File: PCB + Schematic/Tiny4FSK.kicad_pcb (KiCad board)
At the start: 4 copper layers, 30.9 x 65.8 mm, 81 parts, among them IC1 SI4063, J1 SWD, J2 GPIO, J3 USBC, J4 OPTIONAL, J5 I2C, J6 Power, J7 SPI, SW1 RST, SW2 BATT PWR, U1 BME280, U2 MAX-M10S, U3 Linear Step-Down, U4 ATSAMD21G18A-A, U5 TCXO MCU, U6 TPS61200DRC

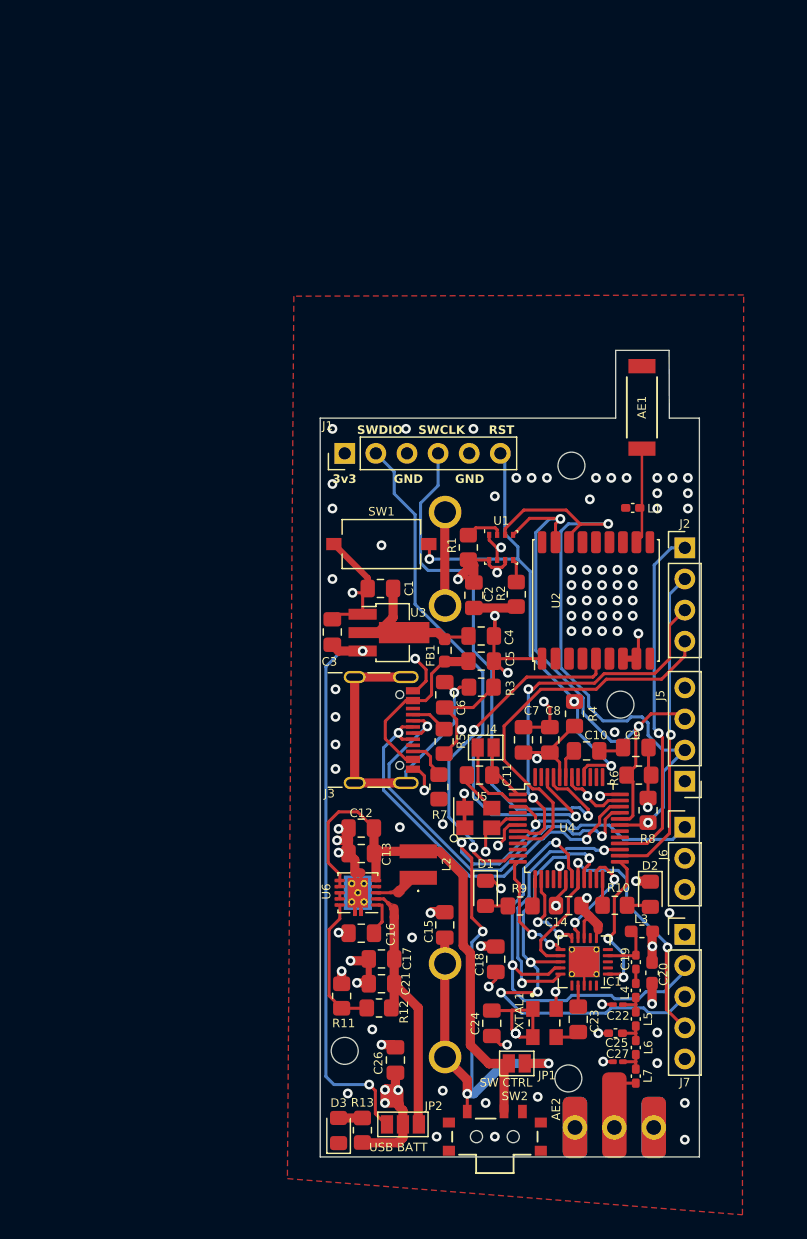
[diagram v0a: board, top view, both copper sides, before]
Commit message: Rebase Rev. 4 PCB files
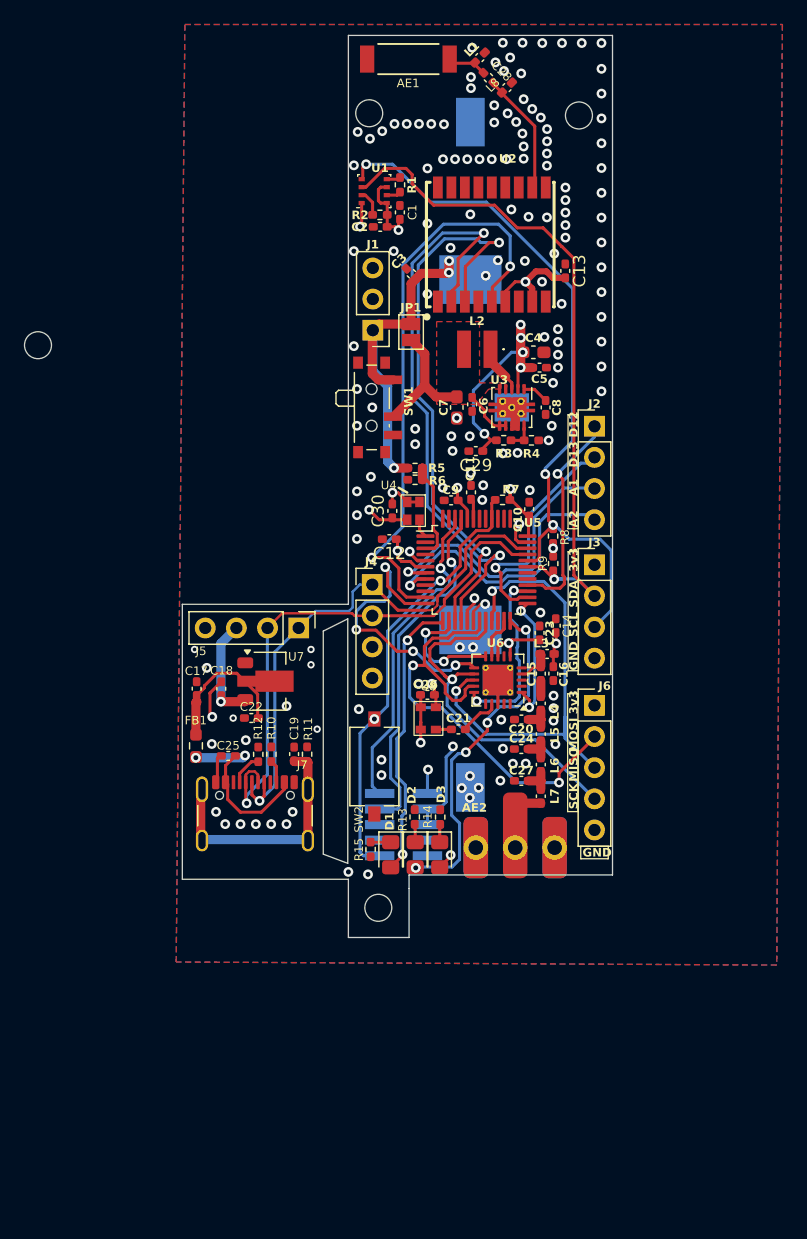
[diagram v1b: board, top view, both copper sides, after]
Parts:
- removed the C11 at (151.0, 99.8)
- removed the C15 at (148.2, 112.0)
- removed the C26 at (144.1, 123.0)
- removed the C4 at (151.1, 88.4)
- removed the C5 at (151.1, 90.5)
- removed the C6 at (148.2, 93.2)
- removed the G*** at (151.2, 102.8)
- removed the G*** at (151.1, 90.5)
- removed the G*** at (142.5, 127.5)
- removed the G*** at (153.0, 127.5)
- removed the J1 at (140.0, 73.5)
- removed JP2: Source, Jumper:SolderJumper-3_P1.3mm_Open_Pad1.0x1.5mm_NumberLabels
- removed the R3 at (151.1, 92.6)
- removed the R7 at (147.7, 100.7)
- removed the U3 at (143.9, 88.1)
- added C13: 100nF, Capacitor_SMD:C_0402_1005Metric_Pad0.74x0.62mm_HandSolder, F.Cu at (158.0, 58.6)
- added C17: 100 nF, Capacitor_SMD:C_0402_1005Metric_Pad0.74x0.62mm_HandSolder, F.Cu at (127.9, 92.7)
- added C18: 1uF, Capacitor_SMD:C_0402_1005Metric_Pad0.74x0.62mm_HandSolder, F.Cu at (129.9, 92.7)
- added C19: 4.7 nF, Capacitor_SMD:C_0402_1005Metric_Pad0.74x0.62mm_HandSolder, F.Cu at (135.9, 98.0)
- added C22: 1uF, Capacitor_SMD:C_0402_1005Metric_Pad0.74x0.62mm_HandSolder, F.Cu at (132.4, 95.1)
- added C25: 100 nF, Capacitor_SMD:C_0402_1005Metric_Pad0.74x0.62mm_HandSolder, F.Cu at (130.5, 98.2)
- added C28: 1.5pF, Capacitor_SMD:C_0402_1005Metric_Pad0.74x0.62mm_HandSolder, F.Cu at (151.7, 42.9)
- added C29: 100nF, Capacitor_SMD:C_0402_1005Metric_Pad0.74x0.62mm_HandSolder, F.Cu at (150.7, 73.3)
- added C30: 100 nF, Capacitor_SMD:C_0402_1005Metric_Pad0.74x0.62mm_HandSolder, F.Cu at (143.9, 78.2)
- added G***: LOGO, LOGO, B.Cu at (144.4, 41.0)
- added G***: LOGO, LOGO, B.Cu at (149.1, 80.1)
- added G***: LOGO, LOGO, B.Cu at (159.3, 41.5)
- added G***: LOGO, LOGO, B.Cu at (149.1, 67.5)
- added G***: LOGO, LOGO, B.Cu at (144.7, 43.1)
- added G***: LOGO, LOGO, B.Cu at (144.7, 45.4)
- added J6: SPI, Connector_PinHeader_2.54mm:PinHeader_1x05_P2.54mm_Vertical, F.Cu at (160.4, 94.1)
- added J8: SWD, Connector_PinHeader_1.27mm:PinHeader_2x05_P1.27mm_Vertical_SMD, B.Cu at (144.8, 103.8)
- added L8: 3.9 nH, Inductor_SMD:L_0402_1005Metric_Pad0.77x0.64mm_HandSolder, F.Cu at (153.2, 43.7)
- added R10: 5k1, Resistor_SMD:R_0402_1005Metric_Pad0.72x0.64mm_HandSolder, F.Cu at (134.0, 98.0)
- added R11: 1M, Resistor_SMD:R_0402_1005Metric_Pad0.72x0.64mm_HandSolder, F.Cu at (136.9, 98.0)
- added R12: 5k1, Resistor_SMD:R_0402_1005Metric_Pad0.72x0.64mm_HandSolder, F.Cu at (132.9, 98.1)
- added R6: 1M, Resistor_SMD:R_0402_1005Metric_Pad0.72x0.64mm_HandSolder, F.Cu at (145.7, 75.7)
- added U7: Linear Step-Down, LDO:MCP1700, F.Cu at (133.5, 92.1)
- AE1: value GPS ANT -> 1575AT43A0040
- AE2: value ANT -> TX Antenna
- BT1: value AAA -> BK-53; footprint BatteryExtended:BAT_BK-82 -> BatteryExtended:BAT_53
- C1: value 1uF -> 10uF; footprint Capacitor_SMD:C_0805_2012Metric_Pad1.18x1.45mm_HandSolder -> Capacitor_SMD:C_0402_1005Metric_Pad0.74x0.62mm_HandSolder
- C10: renamed from C9; value 100nF -> 100 nF; footprint Capacitor_SMD:C_0805_2012Metric_Pad1.18x1.45mm_HandSolder -> Capacitor_SMD:C_0402_1005Metric_Pad0.74x0.62mm_HandSolder
- C11: renamed from C10; footprint Capacitor_SMD:C_0805_2012Metric_Pad1.18x1.45mm_HandSolder -> Capacitor_SMD:C_0402_1005Metric_Pad0.74x0.62mm_HandSolder
- C12: renamed from C7; value 100nF -> 10 uF; footprint Capacitor_SMD:C_0805_2012Metric_Pad1.18x1.45mm_HandSolder -> Capacitor_SMD:C_0402_1005Metric_Pad0.74x0.62mm_HandSolder
- C14, C2, C3: footprint Capacitor_SMD:C_0805_2012Metric_Pad1.18x1.45mm_HandSolder -> Capacitor_SMD:C_0402_1005Metric_Pad0.74x0.62mm_HandSolder
- C16: renamed from C20; footprint Capacitor_SMD:C_0603_1608Metric_Pad1.08x0.95mm_HandSolder -> Capacitor_SMD:C_0402_1005Metric_Pad0.74x0.62mm_HandSolder
- C20: renamed from C22; value 15 pF -> 8 pF; footprint Capacitor_SMD:C_0201_0603Metric_Pad0.64x0.40mm_HandSolder -> Capacitor_SMD:C_0402_1005Metric_Pad0.74x0.62mm_HandSolder
- C21: renamed from C23; footprint Capacitor_SMD:C_0805_2012Metric_Pad1.18x1.45mm_HandSolder -> Capacitor_SMD:C_0402_1005Metric_Pad0.74x0.62mm_HandSolder
- C23: renamed from C18; footprint Capacitor_SMD:C_0805_2012Metric_Pad1.18x1.45mm_HandSolder -> Capacitor_SMD:C_0402_1005Metric_Pad0.74x0.62mm_HandSolder
- C24: renamed from C25; value 12 pF -> 6 pF
- C26: renamed from C24; value 10 nF -> 100 nF; footprint Capacitor_SMD:C_0805_2012Metric_Pad1.18x1.45mm_HandSolder -> Capacitor_SMD:C_0402_1005Metric_Pad0.74x0.62mm_HandSolder
- C27: value 10 pF -> 5 pF; footprint Capacitor_SMD:C_0201_0603Metric_Pad0.64x0.40mm_HandSolder -> Capacitor_SMD:C_0402_1005Metric_Pad0.74x0.62mm_HandSolder
- C4: renamed from C17; footprint Capacitor_SMD:C_0805_2012Metric_Pad1.18x1.45mm_HandSolder -> Capacitor_SMD:C_0603_1608Metric_Pad1.08x0.95mm_HandSolder
- C5: renamed from C21; footprint Capacitor_SMD:C_0805_2012Metric_Pad1.18x1.45mm_HandSolder -> Capacitor_SMD:C_0402_1005Metric_Pad0.74x0.62mm_HandSolder
- C6: renamed from C12; value 10uF -> 100 nF; footprint Capacitor_SMD:C_0805_2012Metric_Pad1.18x1.45mm_HandSolder -> Capacitor_SMD:C_0402_1005Metric_Pad0.74x0.62mm_HandSolder
- C7: renamed from C13; value 100nF -> 10 uF; footprint Capacitor_SMD:C_0805_2012Metric_Pad1.18x1.45mm_HandSolder -> Capacitor_SMD:C_0603_1608Metric_Pad1.08x0.95mm_HandSolder
- C8: renamed from C16; footprint Capacitor_SMD:C_0805_2012Metric_Pad1.18x1.45mm_HandSolder -> Capacitor_SMD:C_0402_1005Metric_Pad0.74x0.62mm_HandSolder
- C9: renamed from C8; footprint Capacitor_SMD:C_0805_2012Metric_Pad1.18x1.45mm_HandSolder -> Capacitor_SMD:C_0402_1005Metric_Pad0.74x0.62mm_HandSolder
- J1: renamed from J6; value Power -> Power Ext
- J3: value USBC -> I2C; footprint Connector_USB:USB_C_Receptacle_GCT_USB4105-xx-A_16P_TopMnt_Horizontal -> Connector_PinHeader_2.54mm:PinHeader_1x04_P2.54mm_Vertical
- J4: value OPTIONAL -> USB; footprint Jumper:SolderJumper-2_P1.3mm_Open_Pad1.0x1.5mm -> Connector_PinHeader_2.54mm:PinHeader_1x04_P2.54mm_Vertical
- J5: value I2C -> USB Breakout
- J7: value SPI -> USBC; footprint Connector_PinHeader_2.54mm:PinHeader_1x05_P2.54mm_Vertical -> Connector_USB:USB_C_Receptacle_GCT_USB4105-xx-A_16P_TopMnt_Horizontal
- JP1: value SWITCH_EN -> Switch EN
- L1: value 33 nH -> 3.9 nH
- L3: footprint Inductor_SMD:L_0603_1608Metric_Pad1.05x0.95mm_HandSolder -> Inductor_SMD:L_0402_1005Metric_Pad0.77x0.64mm_HandSolder
- L4: value 33 nH -> 14 nH
- L5: value 30 nH -> 14 nH
- L6: value 36 nH -> 14 nH
- L7: value 22 nH -> 14 nH
- R1: renamed from R2; footprint Resistor_SMD:R_0805_2012Metric_Pad1.20x1.40mm_HandSolder -> Resistor_SMD:R_0402_1005Metric_Pad0.72x0.64mm_HandSolder
- R13: renamed from R10; value 100 -> 330; footprint Resistor_SMD:R_0805_2012Metric_Pad1.20x1.40mm_HandSolder -> Resistor_SMD:R_0402_1005Metric_Pad0.72x0.64mm_HandSolder
- R14: renamed from R13; value 1k -> 330; footprint Resistor_SMD:R_0805_2012Metric_Pad1.20x1.40mm_HandSolder -> Resistor_SMD:R_0402_1005Metric_Pad0.72x0.64mm_HandSolder
- R15: renamed from R9; value 100 -> 330; footprint Resistor_SMD:R_0805_2012Metric_Pad1.20x1.40mm_HandSolder -> Resistor_SMD:R_0402_1005Metric_Pad0.72x0.64mm_HandSolder
- R2: renamed from R1; footprint Resistor_SMD:R_0805_2012Metric_Pad1.20x1.40mm_HandSolder -> Resistor_SMD:R_0402_1005Metric_Pad0.72x0.64mm_HandSolder
- R3: renamed from R12; value 5M -> 1M; footprint Resistor_SMD:R_0805_2012Metric_Pad1.20x1.40mm_HandSolder -> Resistor_SMD:R_0402_1005Metric_Pad0.72x0.64mm_HandSolder
- R4: renamed from R11; value 900k -> 180k; footprint Resistor_SMD:R_0805_2012Metric_Pad1.20x1.40mm_HandSolder -> Resistor_SMD:R_0402_1005Metric_Pad0.72x0.64mm_HandSolder
- R5: value 5k1 -> 1M; footprint Resistor_SMD:R_0805_2012Metric_Pad1.20x1.40mm_HandSolder -> Resistor_SMD:R_0402_1005Metric_Pad0.72x0.64mm_HandSolder
- R7: renamed from R4; footprint Resistor_SMD:R_0805_2012Metric_Pad1.20x1.40mm_HandSolder -> Resistor_SMD:R_0402_1005Metric_Pad0.72x0.64mm_HandSolder
- R8: renamed from R6; footprint Resistor_SMD:R_0805_2012Metric_Pad1.20x1.40mm_HandSolder -> Resistor_SMD:R_0402_1005Metric_Pad0.72x0.64mm_HandSolder
- R9: renamed from R8; footprint Resistor_SMD:R_0805_2012Metric_Pad1.20x1.40mm_HandSolder -> Resistor_SMD:R_0402_1005Metric_Pad0.72x0.64mm_HandSolder
- SW1: renamed from SW2; value BATT PWR -> Power Switch; footprint SlideSwitch:WS-SLSU_6p7x2p7_WRE -> Button_Switch_SMD:SW_SPDT_PCM12
- U2: value MAX-M10S -> ATGM336H; footprint RF_GPS:ublox_MAX -> RF_GPS_Extended:ATGM336H
- U4: renamed from U5; value TCXO MCU -> ECS-327TXO-2012; footprint Oscillator_TCXO:ATXK-H11-E-32.768KHZ-E50-T3 -> Oscillator_TCXO:ECS-327TXO-2012
- U8: renamed from XTAL1; footprint OSC:OSC_ECS-TXO-32CSMV-260-AN-TR -> Oscillator_TCXO:ECS-TXO-20CSMV4
- moved H3 62.8 mm to (115.0, 64.7)
- moved JP1 60.3 mm to (145.4, 63.6), turned to 90 degrees
- moved SW1 60.3 mm to (142.5, 69.8), turned to -90 degrees
- moved C5 51.9 mm to (155.9, 66.5), turned to 0 degrees
- moved C4 51.0 mm to (155.4, 65.3), turned to 0 degrees
- moved H2 48.2 mm to (159.1, 45.9)
- moved R4 47.9 mm to (155.2, 72.4), turned to 0 degrees
- moved J1 47.9 mm to (142.3, 63.5), turned to 180 degrees
- moved R3 47.4 mm to (153.0, 72.4), turned to 0 degrees
- moved C8 45.5 mm to (156.4, 69.8), turned to -90 degrees
- moved BT1 44.3 mm to (150.2, 74.9), turned to -90 degrees
- moved L2 42.3 mm to (150.8, 65.0), turned to 180 degrees
- moved U3 41.5 mm to (153.6, 69.8), turned to -90 degrees
- moved L1 38.8 mm to (151.0, 41.2), turned to -135 degrees
- moved C7 37.2 mm to (149.1, 69.8), turned to -90 degrees
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- renumbered C19 to C15, SW1 to SW2, U6 to U3, U4 to U5, IC1 to U6
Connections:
- net EXTINT renamed GPS_EN
- AE1 pad 1: ANT_GPS -> Net-(AE1-A)
- C1 pad 2: LIN -> +3.3V
- C3 pad 1: LDO -> +BATT
- C4 pad 1: BOOST -> +3.3V
- C5 pad 1: BOOST -> +3.3V
- D1 pad 1: Earth -> Net-(D1-K)
- D1 pad 2: Net-(D1-A) -> SUCCESS
- D2 pad 1: Earth -> Net-(D2-K)
- D2 pad 2: Net-(D2-A) -> ERROR
- D3 pad 1: Earth -> Net-(D3-K)
- D3 pad 2: Net-(D3-A) -> +3.3V
- J1 pad 1: BATT_SENSE -> +BATT
- J4 pad 1: TCXO -> D+
- J4 pad 2: OPT XOUT -> D-
- J5 pad 1: +3.3V -> D+
- J5 pad 2: SDA -> D-
- J5 pad 3: SCL -> +3.3V
- JP1 pad 2: BATT_SENSE -> +BATT
- L1 pad 2: ANT_GPS -> Net-(AE1-A)
- R13 pad 1: ERROR -> Net-(D2-K)
- R13 pad 2: Net-(D2-A) -> Earth
- R14 pad 1: +3.3V -> Net-(D3-K)
- R14 pad 2: Net-(D3-A) -> Earth
- R15 pad 1: Net-(D1-A) -> Net-(D1-K)
- R15 pad 2: SUCCESS -> Earth
- R3 pad 1: BOOST -> +3.3V
- R5 pad 1: Earth -> +BATT
- R5 pad 2: Net-(J3-CC1) -> BATT_SENSE
- R8 pad 1: SCL -> +3.3V
- R8 pad 2: +3.3V -> SCL
- SW1 pad 1: BATT_SENSE -> +BATT
- U2 pad 16: SDA -> unconnected-(U2-SDA-Pad16)
- U2 pad 17: SCL -> unconnected-(U2-SCL-Pad17)
- U2 pad 2: unconnected-(U2-TXD-Pad2) -> RXD
- U2 pad 3: unconnected-(U2-RXD-Pad3) -> TXD
- U2 pad 6: unconnected-(U2-V_BCKP-Pad6) -> +3.3V
- U2 pad 7: +3.3V -> unconnected-(U2-NC-Pad7)
- U3 pad 2: BOOST -> +3.3V
- U4 pad 3: Net-(U5-OUTPUT) -> TCXO
- U5 pad 15: unconnected-(U4-PA10-Pad15) -> TXD
- U5 pad 16: unconnected-(U4-PA11-Pad16) -> RXD
- U5 pad 2: OPT XOUT -> unconnected-(U5-PA01-Pad2)
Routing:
- net Earth: track 106.9 -> 36.0 mm, vias 95 -> 150
- net BATT_SENSE: track 70.9 -> 8.07 mm, vias 5 -> 0
- net RXD: track 0.00 -> 48.7 mm, vias 0 -> 2
- net LDO: track 47.4 -> 0.00 mm, vias 2 -> 0
- net TXD: track 0.00 -> 46.7 mm, vias 0 -> 2
- net BST_IN: track 45.1 -> 14.8 mm
- net +BATT: track 0.00 -> 30.2 mm, vias 0 -> 5
- net Net-(J3-SHIELD): track 28.6 -> 0.00 mm, vias 1 -> 0
- net ERROR: track 2.14 -> 28.3 mm, vias 0 -> 4
- net BOOST: track 22.1 -> 0.00 mm
- net SUCCESS: track 1.96 -> 23.4 mm, vias 0 -> 2
- net Net-(J7-SHIELD): track 0.00 -> 19.9 mm
- net GPS_EN: track 28.8 -> 48.2 mm
- net SWDIO: track 45.2 -> 26.4 mm
- net SWCLK: track 45.9 -> 28.7 mm
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- added copper zone on F.Cu, net BST_IN
- added copper zone on B.Cu, net Earth
- removed copper zone on F.Cu, net BOOST
- removed copper zone on F.Cu, net Net-(U3-L)
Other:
- board size 30.9 x 65.8 mm -> 35.1 x 73.6 mm
- board text added: "Licensed under CERN-OHL-W-2.0"
- board text added: "Made by Max Kendall, W0MXX"
- board text added: "Max W0MXX"
- board text added: "November 2024"
- board text added: "Rev. 4.0"
- board text added: "Sponsored by:"
- board text added: "USB Breakout"
- board text added: "WayWayWay"
- board text removed: "+"
- board text removed: "-"
- board text removed: "BST"
- board text removed: "Developed by Max W0MXX"
- board text removed: "JP1 - Cut to enable SW2 for PWR JP2 - Control PWR source (USB and CTR for USB, CTR and BATT) SW1 - RST SW2 - BATT PWR AE2 - 70cm ANT"
- board text removed: "RST"
- board text removed: "Rev. 3 - 4/19/24"
- board text removed: "SW CTRL"
- board text removed: "SWCLK"
- board text removed: "SWDIO"
- board text removed: "USB BATT"
